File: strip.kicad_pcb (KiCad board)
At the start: 4 copper layers, 66 x 18 mm, 43 parts, among them J105 CORTEX-DEBUG, J106 JAE_DX07S016JA3, J301 WAGO-2065, J302 WAGO-2065, J303 WAGO-2065, SW101 SW_Push, SW102 SW_Push, U102 ATSAMD51G, U103 AP2112K-3.3, U301 74AHC1G125, Y101 32k768

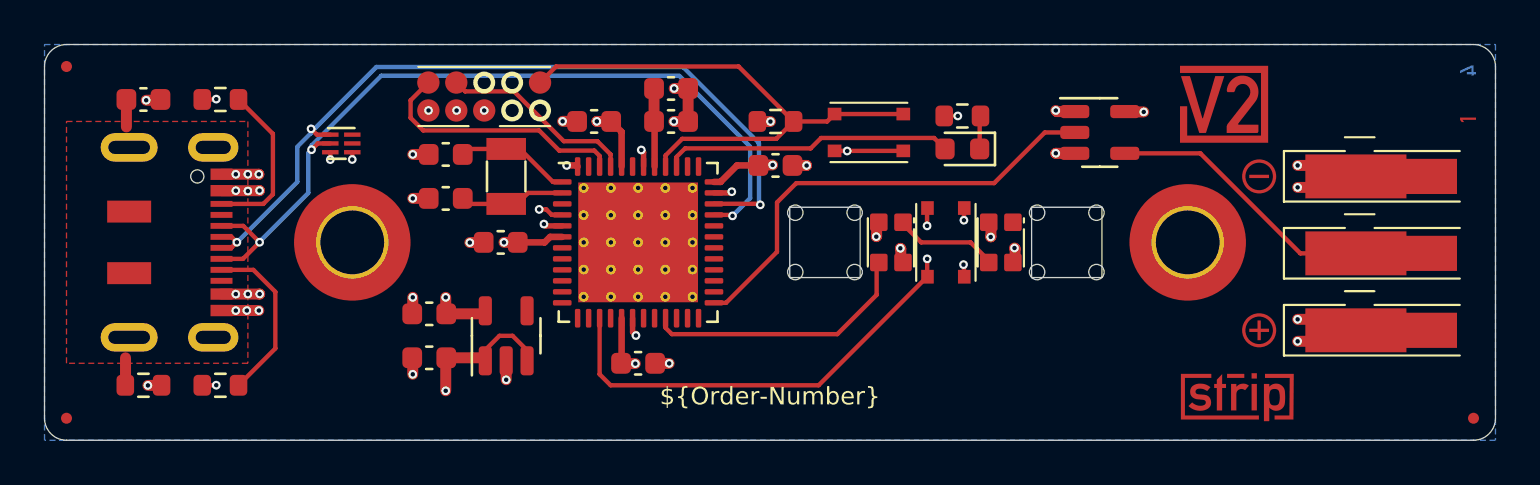
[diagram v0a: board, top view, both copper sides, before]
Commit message: Refresh
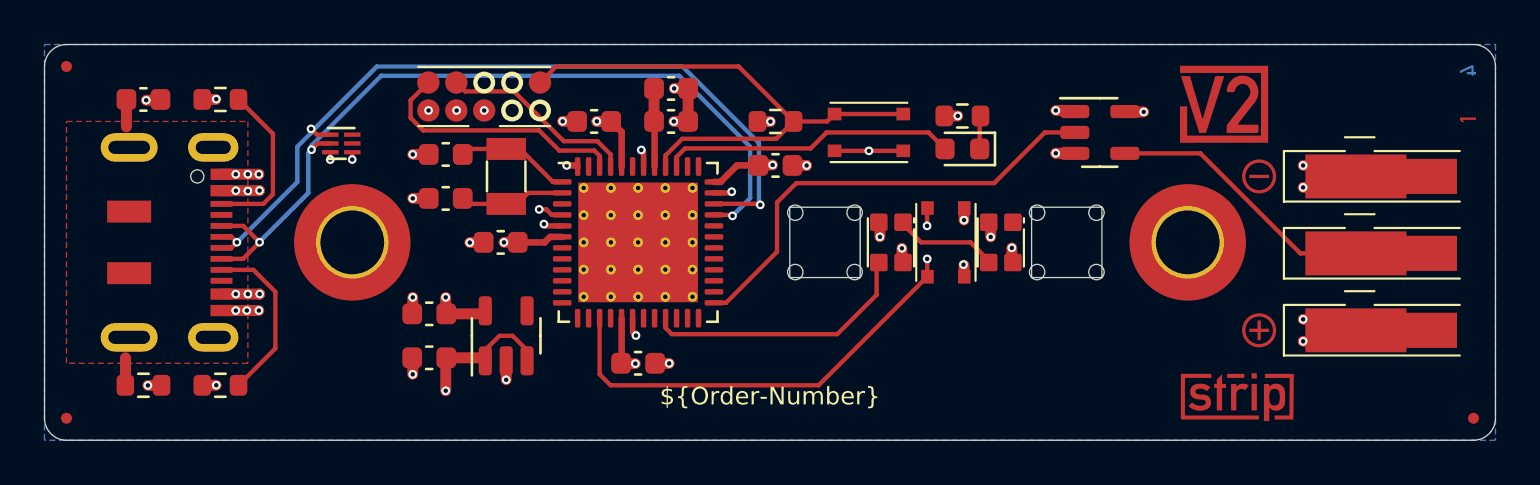
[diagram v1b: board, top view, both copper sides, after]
